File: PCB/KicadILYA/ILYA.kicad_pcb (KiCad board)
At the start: 2 copper layers, 6 parts

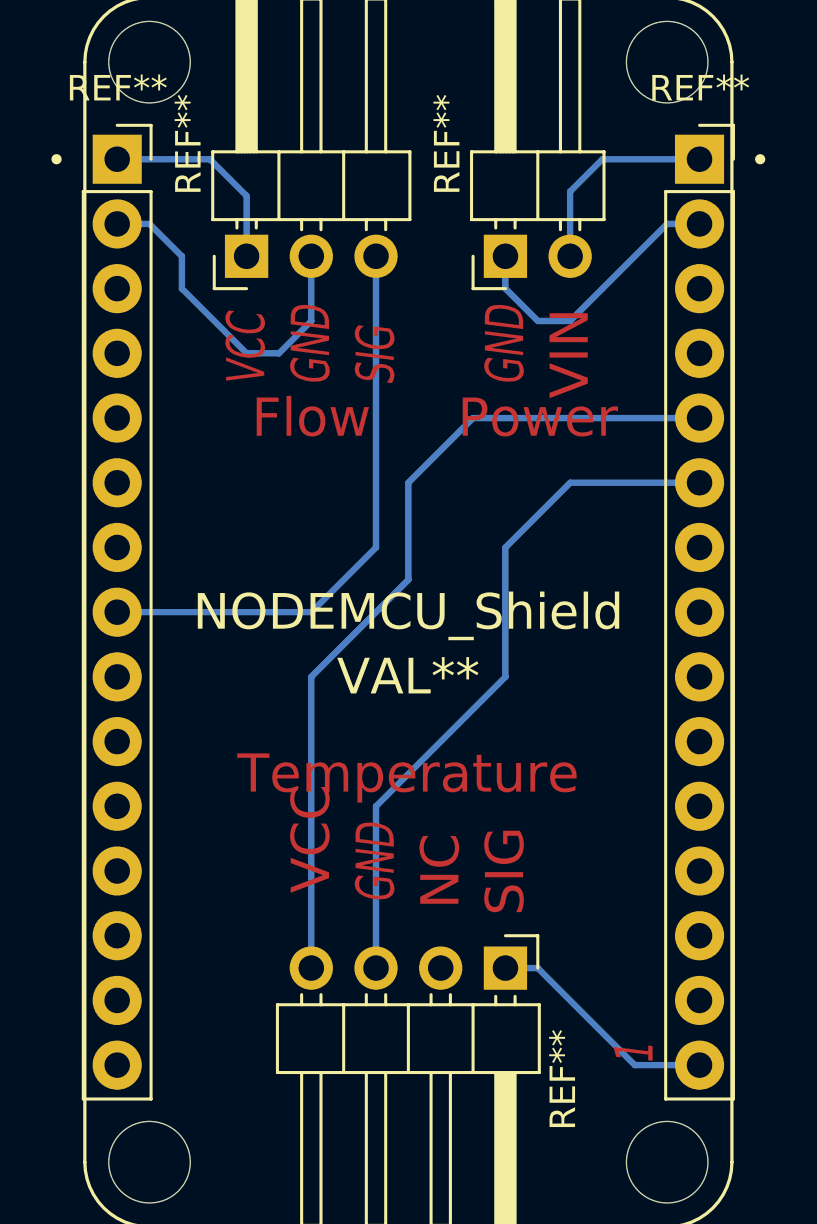
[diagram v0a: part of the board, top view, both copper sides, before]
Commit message: PCB NODEMCU + PCB WEMOS
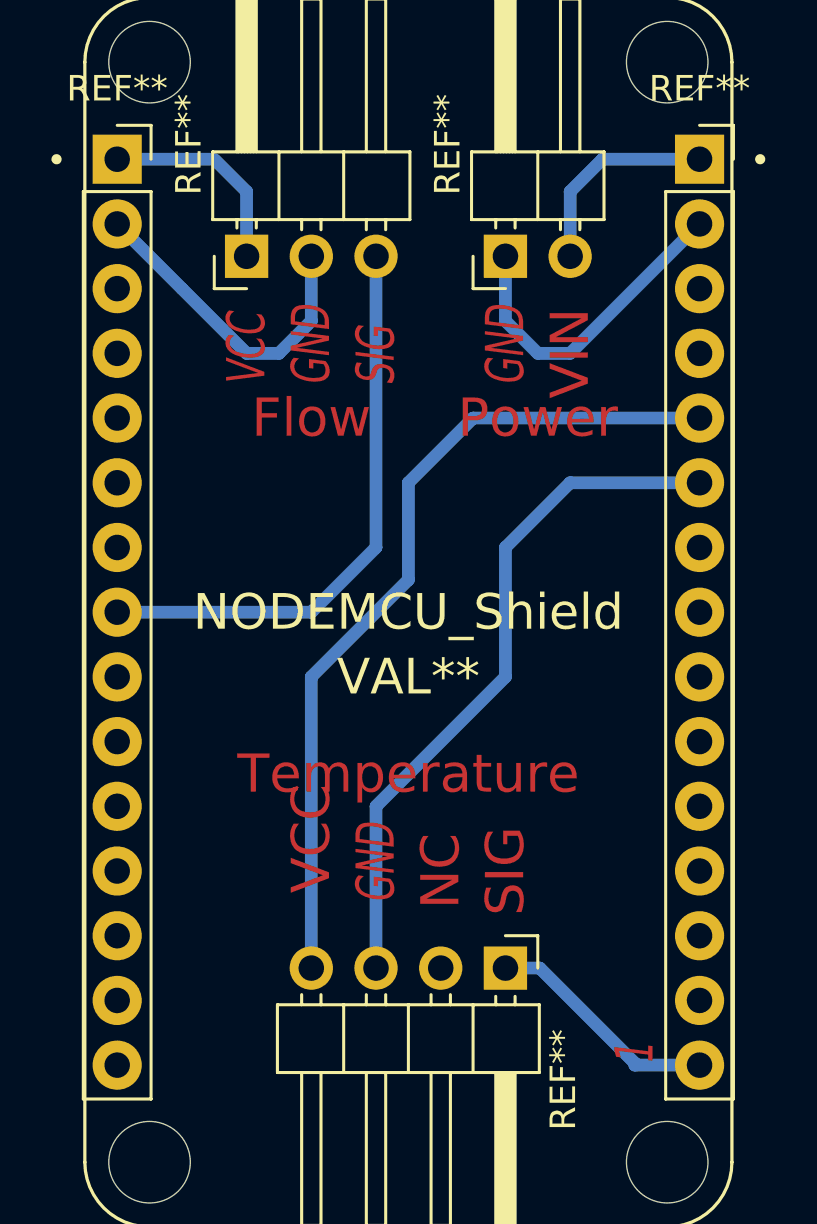
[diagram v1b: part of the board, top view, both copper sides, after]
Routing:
- net (no net): track 133.0 -> 135.3 mm
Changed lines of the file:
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@@
     (thickness 1.6)
     (drawings 13)
-    (tracks 35)
+    (tracks 33)
     (zones 0)
     (modules 6)
@@
     (pad_drill 0.6)
     (pad_to_mask_clearance 0)
+    (solder_mask_min_width 0.25)
     (aux_axis_origin 0 0)
     (visible_elements FFFFF77F)
@@
     (effects (font (size 1.5 1.5) (thickness 0.3)))
   )
-  (segment (start 116.84 97.79) (end 114.3 100.33) (width 0.25) (layer B.Cu) (net 0))
-  (segment (start 114.3 100.33) (end 106.68 100.33) (width 0.25) (layer B.Cu) (net 0))
-  (segment (start 120.65 92.71) (end 129.54 92.71) (width 0.25) (layer B.Cu) (net 0))
-  (segment (start 118.11 99.06) (end 118.11 95.25) (width 0.25) (layer B.Cu) (net 0))
-  (segment (start 118.11 95.25) (end 120.65 92.71) (width 0.25) (layer B.Cu) (net 0))
-  (segment (start 114.3 102.87) (end 118.11 99.06) (width 0.25) (layer B.Cu) (net 0))
-  (segment (start 116.84 107.95) (end 121.92 102.87) (width 0.25) (layer B.Cu) (net 0))
-  (segment (start 121.92 102.87) (end 121.92 97.79) (width 0.25) (layer B.Cu) (net 0))
-  (segment (start 124.46 95.25) (end 129.54 95.25) (width 0.25) (layer B.Cu) (net 0))
-  (segment (start 121.92 97.79) (end 124.46 95.25) (width 0.25) (layer B.Cu) (net 0))
-  (segment (start 116.84 114.3) (end 116.84 107.95) (width 0.25) (layer B.Cu) (net 0))
-  (segment (start 114.3 114.3) (end 114.3 102.87) (width 0.25) (layer B.Cu) (net 0))
-  (segment (start 110.32 82.55) (end 111.76 83.99) (width 0.25) (layer B.Cu) (net 0))
-  (segment (start 106.68 82.55) (end 110.32 82.55) (width 0.25) (layer B.Cu) (net 0))
-  (segment (start 129.54 82.55) (end 125.73 82.55) (width 0.25) (layer B.Cu) (net 0))
-  (segment (start 125.73 82.55) (end 124.46 83.82) (width 0.25) (layer B.Cu) (net 0))
-  (segment (start 129.54 85.09) (end 128.27 85.09) (width 0.25) (layer B.Cu) (net 0))
-  (segment (start 128.27 85.09) (end 125.73 87.63) (width 0.25) (layer B.Cu) (net 0))
-  (segment (start 123.19 114.3) (end 121.92 114.3) (width 0.25) (layer B.Cu) (net 0))
-  (segment (start 129.54 118.11) (end 127 118.11) (width 0.25) (layer B.Cu) (net 0))
-  (segment (start 127 118.11) (end 123.19 114.3) (width 0.25) (layer B.Cu) (net 0))
-  (segment (start 124.46 86.36) (end 124.46 83.82) (width 0.25) (layer B.Cu) (net 0))
-  (segment (start 125.73 87.63) (end 124.46 88.9) (width 0.25) (layer B.Cu) (net 0))
+  (segment (start 106.68 82.55) (end 110.32 82.55) (width 0.5) (layer B.Cu) (net 0))
   (segment (start 121.92 86.36) (end 121.92 87.63) (width 0.25) (layer B.Cu) (net 0))
-  (segment (start 121.92 87.63) (end 123.19 88.9) (width 0.25) (layer B.Cu) (net 0))
-  (segment (start 123.19 88.9) (end 124.46 88.9) (width 0.25) (layer B.Cu) (net 0))
-  (segment (start 111.76 83.99) (end 111.76 86.36) (width 0.25) (layer B.Cu) (net 0))
-  (segment (start 116.84 86.36) (end 116.84 97.79) (width 0.25) (layer B.Cu) (net 0))
-  (segment (start 114.3 86.36) (end 114.3 88.9) (width 0.25) (layer B.Cu) (net 0))
-  (segment (start 114.3 88.9) (end 113.03 90.17) (width 0.25) (layer B.Cu) (net 0))
-  (segment (start 113.03 90.17) (end 111.76 90.17) (width 0.25) (layer B.Cu) (net 0))
-  (segment (start 111.76 90.17) (end 109.22 87.63) (width 0.25) (layer B.Cu) (net 0))
-  (segment (start 109.22 87.63) (end 109.22 86.36) (width 0.25) (layer B.Cu) (net 0))
-  (segment (start 109.22 86.36) (end 107.95 85.09) (width 0.25) (layer B.Cu) (net 0))
-  (segment (start 107.95 85.09) (end 106.68 85.09) (width 0.25) (layer B.Cu) (net 0))
+  (segment (start 111.76 86.36) (end 111.76 83.82) (width 0.5) (layer B.Cu) (net 0))
+  (segment (start 111.76 83.82) (end 110.49 82.55) (width 0.5) (layer B.Cu) (net 0))
+  (segment (start 124.46 86.36) (end 124.46 83.82) (width 0.5) (layer B.Cu) (net 0))
+  (segment (start 125.73 82.55) (end 124.46 83.82) (width 0.5) (layer B.Cu) (net 0))
+  (segment (start 129.54 82.55) (end 125.73 82.55) (width 0.5) (layer B.Cu) (net 0))
+  (segment (start 129.54 85.09) (end 124.46 90.17) (width 0.5) (layer B.Cu) (net 0))
+  (segment (start 123.19 90.17) (end 124.46 90.17) (width 0.5) (layer B.Cu) (net 0))
+  (segment (start 121.92 88.9) (end 121.92 86.36) (width 0.5) (layer B.Cu) (net 0))
+  (segment (start 123.19 90.17) (end 121.92 88.9) (width 0.5) (layer B.Cu) (net 0))
+  (segment (start 129.54 118.11) (end 127 118.11) (width 0.5) (layer B.Cu) (net 0))
+  (segment (start 127 118.03) (end 127 118.11) (width 0.5) (layer B.Cu) (net 0))
+  (segment (start 123.27 114.3) (end 127 118.03) (width 0.5) (layer B.Cu) (net 0))
+  (segment (start 121.92 114.3) (end 123.27 114.3) (width 0.5) (layer B.Cu) (net 0))
+  (segment (start 114.3 86.36) (end 114.3 88.9) (width 0.5) (layer B.Cu) (net 0))
+  (segment (start 114.3 88.9) (end 113.03 90.17) (width 0.5) (layer B.Cu) (net 0))
+  (segment (start 111.76 90.17) (end 113.03 90.17) (width 0.5) (layer B.Cu) (net 0))
+  (segment (start 109.22 87.63) (end 111.76 90.17) (width 0.5) (layer B.Cu) (net 0))
+  (segment (start 109.22 87.63) (end 106.68 85.09) (width 0.5) (layer B.Cu) (net 0))
+  (segment (start 116.84 97.79) (end 114.3 100.33) (width 0.5) (layer B.Cu) (net 0))
+  (segment (start 116.84 86.36) (end 116.84 97.79) (width 0.5) (layer B.Cu) (net 0))
+  (segment (start 114.3 100.33) (end 106.68 100.33) (width 0.5) (layer B.Cu) (net 0))
+  (segment (start 120.65 92.71) (end 129.54 92.71) (width 0.5) (layer B.Cu) (net 0))
+  (segment (start 120.65 92.71) (end 118.11 95.25) (width 0.5) (layer B.Cu) (net 0))
+  (segment (start 118.11 99.06) (end 118.11 95.25) (width 0.5) (layer B.Cu) (net 0))
+  (segment (start 118.11 99.06) (end 114.3 102.87) (width 0.5) (layer B.Cu) (net 0))
+  (segment (start 114.3 102.87) (end 114.3 114.3) (width 0.5) (layer B.Cu) (net 0))
+  (segment (start 116.84 114.3) (end 116.84 107.95) (width 0.5) (layer B.Cu) (net 0))
+  (segment (start 116.84 107.95) (end 121.92 102.87) (width 0.5) (layer B.Cu) (net 0))
+  (segment (start 121.92 102.87) (end 121.92 97.79) (width 0.5) (layer B.Cu) (net 0))
+  (segment (start 121.92 97.79) (end 124.46 95.25) (width 0.5) (layer B.Cu) (net 0))
+  (segment (start 124.46 95.25) (end 129.54 95.25) (width 0.5) (layer B.Cu) (net 0))
 )

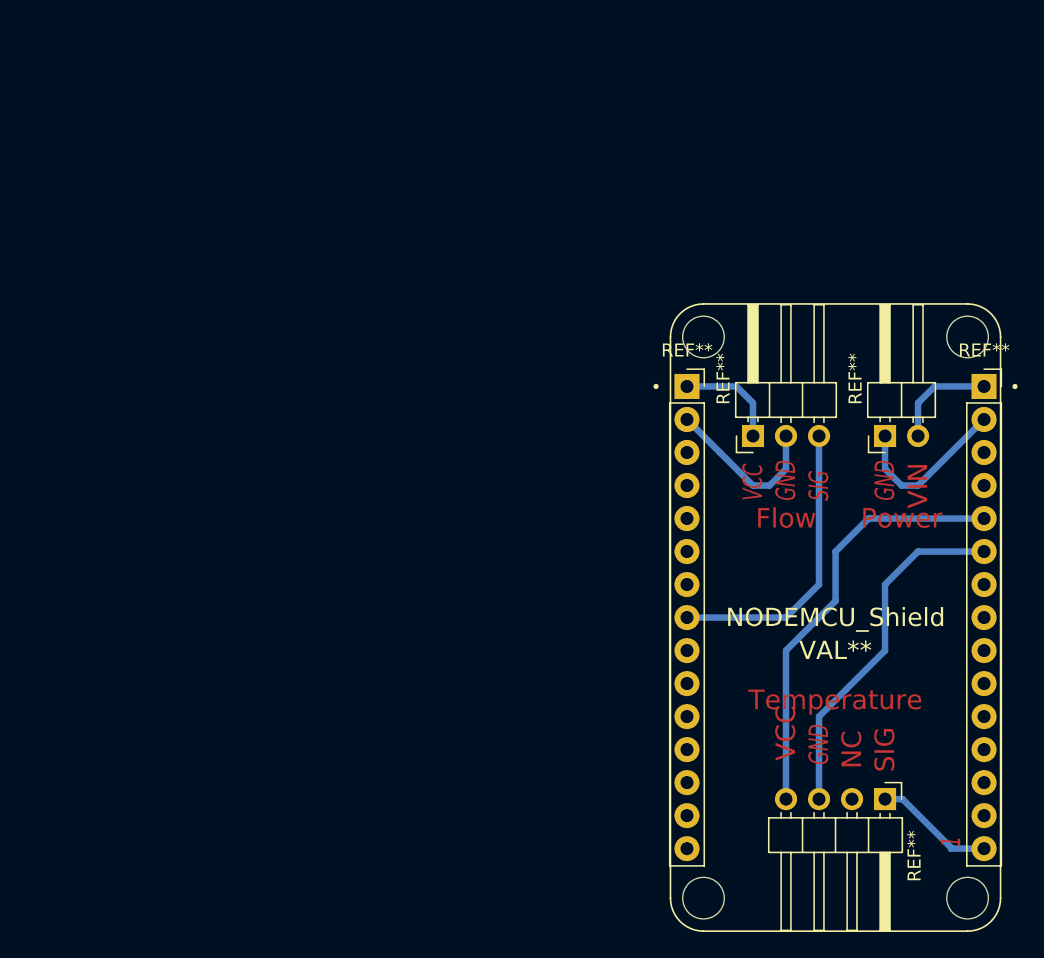
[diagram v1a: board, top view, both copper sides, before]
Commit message: Routage Bon mais connexion pins?
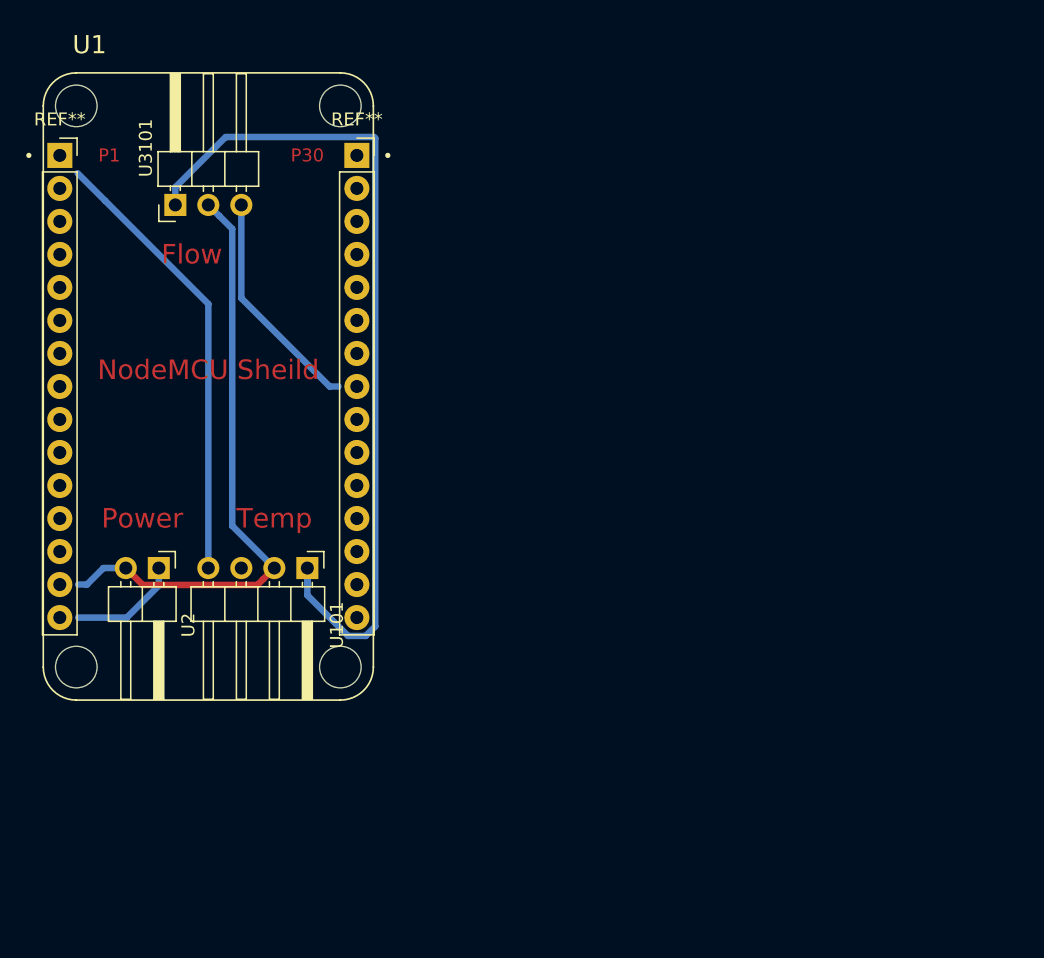
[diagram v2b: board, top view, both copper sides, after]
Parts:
- removed NODEMCU_Shield: VAL**, nodemcu:SEEED_113990105
- removed the REF** at (111.8, 86.4)
- removed the REF** at (129.5, 82.5)
- removed the REF** at (106.7, 82.5)
- removed the REF** at (121.9, 86.4)
- removed the REF** at (121.9, 114.3)
- added REF**: PinSocket_1x15_P2.54mm_Vertical, pinSocket:PinSocket_1x15_P2.54mm_Vertical, F.Cu at (81.3, 64.8)
- added REF**: PinSocket_1x15_P2.54mm_Vertical, pinSocket:PinSocket_1x15_P2.54mm_Vertical, F.Cu at (58.4, 64.8)
- added U1: NodeMCU1.0(ESP-12E), nodemcu:SEEED_113990105, F.Cu at (69.8, 82.5)
- added U101: Temperature_connector, pinHeads:PinHeader_1x04_P2.54mm_Horizontal, F.Cu at (77.5, 96.5)
- added U2: Relay_2_pins, pinHeads:PinHeader_1x02_P2.54mm_Horizontal, F.Cu at (66.0, 96.5)
- added U3101: Flow_connector, pinHeads:PinHeader_1x03_P2.54mm_Horizontal, F.Cu at (67.3, 68.6)
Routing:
- net (no net): track 135.3 -> 0.00 mm
- net VCC: track 0.00 -> 66.2 mm
- net GND: track 0.00 -> 46.7 mm
- net Net-(U1-Pad1): track 0.00 -> 35.0 mm
- net Net-(U1-Pad23): track 0.00 -> 17.5 mm
- net +5V: track 0.00 -> 8.57 mm
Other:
- rule trace_min: 0.2 -> 0.1
- rule via_min_size: 0.4 -> 0.1
- board text added: "NodeMCU Sheild"
- board text added: "P1"
- board text added: "P30"
- board text added: "Temp"
- board text removed: "1"
- board text removed: "GND"
- board text removed: "NC"
- board text removed: "SIG"
- board text removed: "Temperature"
- board text removed: "VCC"
- board text removed: "VIN"
